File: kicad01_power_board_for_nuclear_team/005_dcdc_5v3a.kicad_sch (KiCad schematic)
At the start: 22 parts, among them U501 dcdc_lt8612x

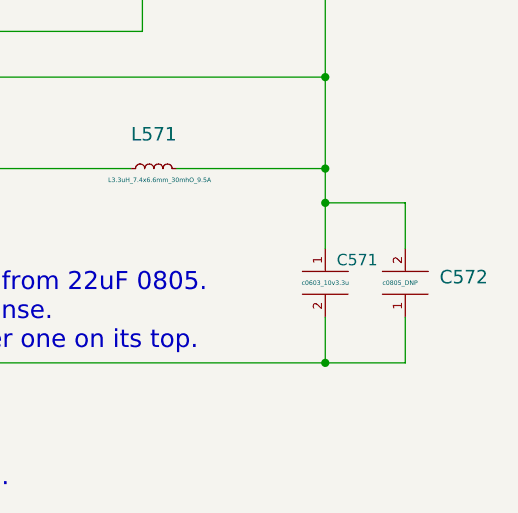
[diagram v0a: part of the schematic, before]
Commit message: x
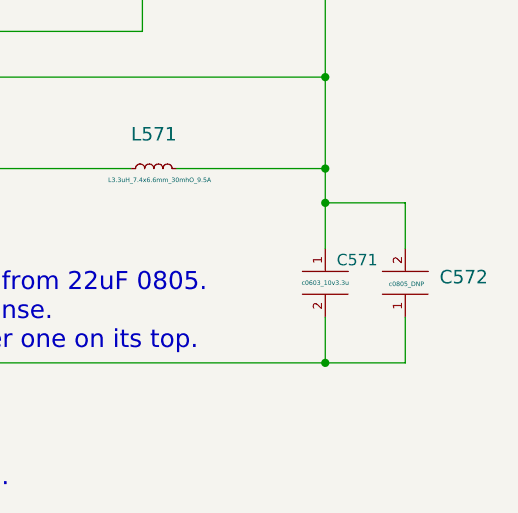
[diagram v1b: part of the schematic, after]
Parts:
- L571: symbol 1001_un:L3.3uH_7.4x6.6mm_30mhO_9.5A -> 1006_Inductance:L3.3uH_7.4x6.6mm_30mhO_9.5A
- U501: symbol 1001_un:dcdc_lt8612x -> 1009_ic:dcdc_lt8612x
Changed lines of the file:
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@@
       (effects (font (size 1.5 1.5)) (justify left))
     )
-    (property "Value" "c0805_DNP" (id 1) (at 224.79 123.19 0)
-      (effects (font (size 0.5 0.5)) (justify left))
+    (property "Value" "c0805_DNP" (id 1) (at 227.457 123.317 0)
+      (effects (font (size 0.5 0.5)))
     )
     (property "Footprint" "02_dyn_pcblib:C0805mix0603" (id 2) (at 228.219 110.363 0)
@@
     (pin "2")
   )
-  (symbol (lib_id "1001_un:L3.3uH_7.4x6.6mm_30mhO_9.5A") (at 199.39 110.49 0) (unit 1)
+  (symbol (lib_id "1006_Inductance:L3.3uH_7.4x6.6mm_30mhO_9.5A") (at 199.39 110.49 0) (unit 1)
     (in_bom yes) (on_board yes)
     (property "Reference" "L571" (id 0) (at 199.39 106.68 0)
@@
     (pin "2")
   )
-  (symbol (lib_id "1001_un:dcdc_lt8612x") (at 120.65 95.25 0) (unit 1)
+  (symbol (lib_id "1009_ic:dcdc_lt8612x") (at 120.65 95.25 0) (unit 1)
     (in_bom yes) (on_board yes)
     (property "Reference" "U501" (id 0) (at 111.76 91.44 0)
